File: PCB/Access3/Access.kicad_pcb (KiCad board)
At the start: 2 copper layers, 57.8 x 27 mm, 76 parts, among them J1 USB-C, J2 RFID, J3 INPUTS, J4 Shelly, J5 POWER, J6 DOOR2, J7 DOOR1, Q1 NX7002AK, Q2 PMF250XNEX, SW1 ESE13V01D, U1 ESP32-PICO-MINI-02, U2 FT231XQ, U3 G3VM-41GR8, U4 LMR16006XDDCR, U5 LMR16006XDDCR, U6 AA, U7 QR, U8 G3VM-41GR8, U9 AA

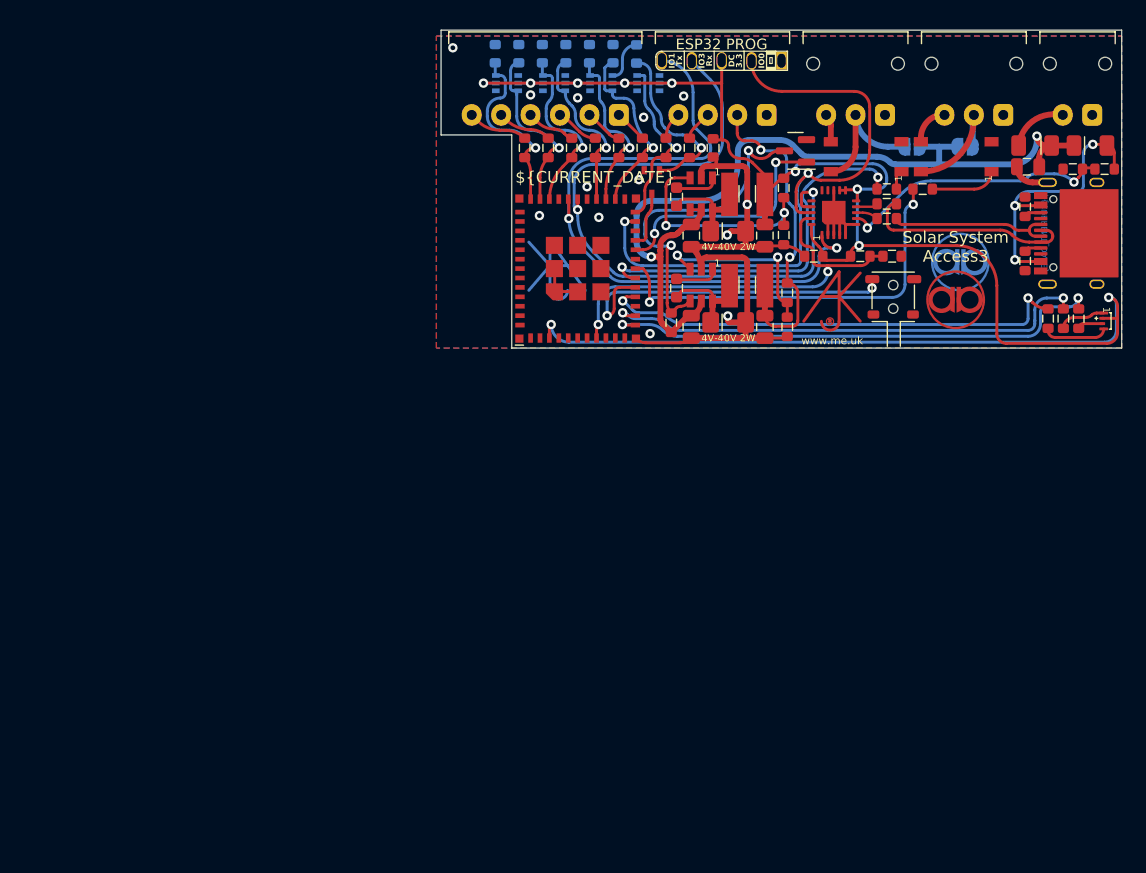
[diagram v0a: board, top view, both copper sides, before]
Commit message: Clean up
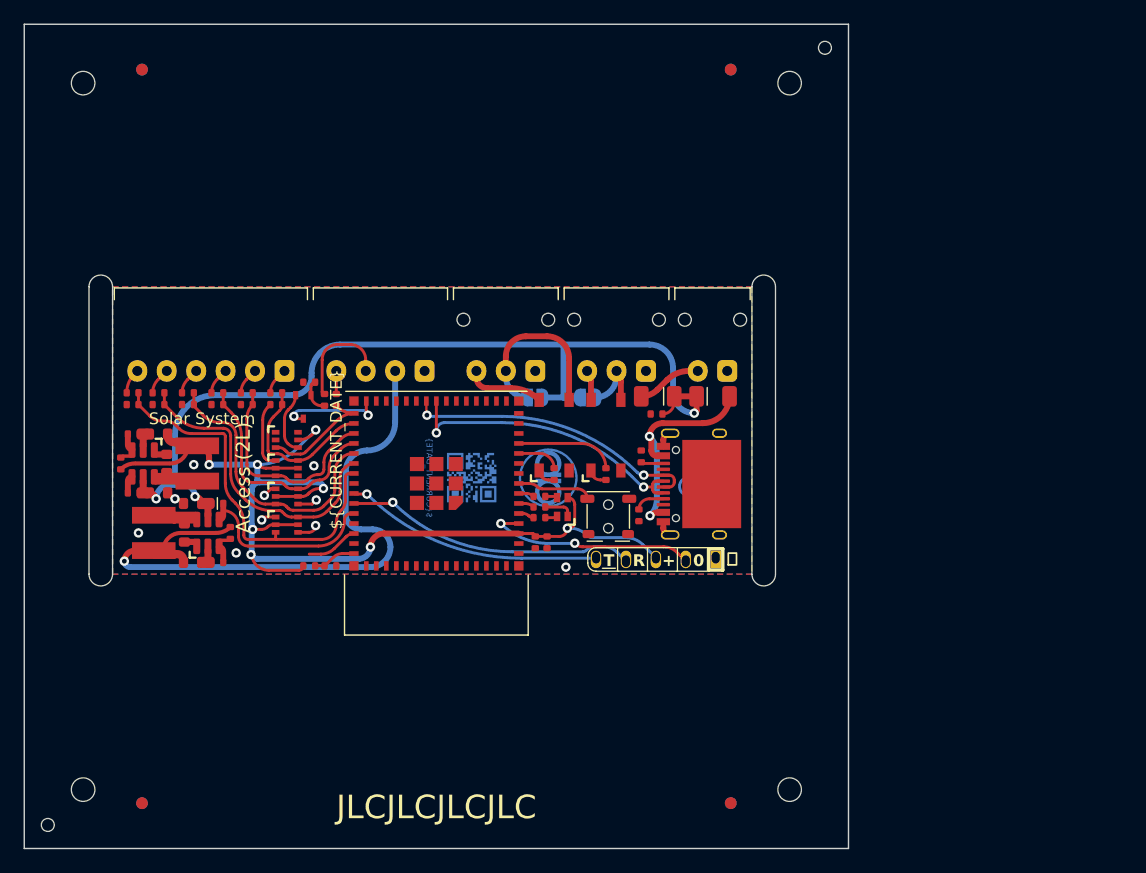
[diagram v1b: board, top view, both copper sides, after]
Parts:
- removed AJK1: AJK, RevK:AJK
- removed C10, C13: 2.2uF, RevK:C_0805_
- removed C11, C14: 10uF, RevK:C_0805_
- removed C12, C9: 100nF, RevK:C_0603_
- removed D5: LED_BARG, RevK:MHS190RGBCT
- removed D7: Schottky, RevK:D_1206_
- removed J4: Shelly, RevK:Shelly
- removed L1, L2: 6.8uH, RevK:L_4x4_
- removed Q1: NX7002AK, Package_TO_SOT_SMD:SOT-23
- removed R17: 300R, RevK:R_0603
- removed R18: 1K, RevK:R_0603
- removed R19: 100R, RevK:R_0603
- removed R22: 100k 1%, RevK:R_0603
- removed R23: 18k 1%, RevK:R_0603
- removed R24: 30k 1%, RevK:R_0603
- removed U4, U5: LMR16006XDDCR, RevK:SOT-23-Thin-6-Reg
- removed U6: AA, RevK:AA
- added C18: 100nF, RevK:C_0402, F.Cu at (108.4, 109.0)
- added C19: 22uF, RevK:C_0402, F.Cu at (109.4, 109.0)
- added C20: 1uF, RevK:C_0402, F.Cu at (91.0, 111.0)
- added C21: 10uF 50V, RevK:C_0603_, F.Cu at (76.6, 104.8)
- added C22: 10uF 6.3V, RevK:C_0603_, F.Cu at (76.4, 99.8)
- added C23: 100nF, RevK:C_0603_, F.Cu at (77.1, 102.3)
- added J8: Shelly, RevK:Shelly, F.Cu at (118.6, 110.5)
- added L3: 10uH, RevK:L_4x4_, F.Cu at (76.0, 108.2)
- added L4: 10uH, RevK:L_4x4_, F.Cu at (79.7, 102.3)
- added PCB1: 70x70, RevK:PCB7070, F.Cu at (100.0, 100.0)
- added R26: 10K, RevK:R_0402, F.Cu at (89.2, 111.0)
- added R27: 1M, RevK:R_0402_, F.Cu at (74.5, 104.8)
- added U10: ESP32-S3-MINI-1, RevK:ESP32-S3-MINI-1, F.Cu at (100.0, 104.0)
- added V1: ~, RevK:VCUT70, F.Cu at (100.0, 87.3)
- added V2: ~, RevK:VCUT70, F.Cu at (100.0, 111.7)
- C1: value 0.1uF -> 10uF 50V; footprint RevK:C_0603 -> RevK:C_0603_
- C15: value 1uF -> 10uF 6.3V; footprint RevK:C_0603 -> RevK:C_0603_
- C16: value 10nF -> 100nF; footprint RevK:C_0603 -> RevK:C_0603_
- C17: footprint RevK:C_0805 -> RevK:C_0402
- C2, C3, C4, C5, C6, C7, C8: footprint RevK:C_0603 -> RevK:C_0402; moved to F.Cu
- D1, D2, D3, D4: footprint Package_TO_SOT_SMD:SOT-363_SC-70-6 -> RevK:SOT-363_SC-70-6; moved to F.Cu
- D6: value Schottky -> RGB; footprint RevK:D_1206_ -> RevK:LED-RGB-1.6x1.6
- Logo1, U9: moved to B.Cu
- R1: value 10k -> 124k; footprint RevK:R_0603 -> RevK:R_0402_
- R10, R11, R12, R13, R16, R25, R4, R5, R6, R7, R8, R9: footprint RevK:R_0603 -> RevK:R_0402
- R14: value 27R -> 124k; footprint RevK:R_0603 -> RevK:R_0402_
- R15: value 27R -> 39k2; footprint RevK:R_0603 -> RevK:R_0402_
- R2: value 4k7 -> 23k2; footprint RevK:R_0603 -> RevK:R_0402_
- R20: value 100K -> 2K; footprint RevK:R_0603 -> RevK:R_0402
- R21: value 100k 1% -> 220R; footprint RevK:R_0603 -> RevK:R_0402
- R3: value 10k -> 680R; footprint RevK:R_0603 -> RevK:R_0402
- U1: value ESP32-PICO-MINI-02 -> MD8942; footprint RevK:ESP32-PICO-MINI-02 -> RevK:SOT-23-6-MD8942
- U2: value FT231XQ -> MD8942; footprint RevK:QFN-20-1EP_4x4mm_P0.5mm_EP2.5x2.5mm -> RevK:SOT-23-6-MD8942
- moved R2 82.4 mm to (81.4, 110.7)
- moved R14 68.7 mm to (73.2, 102.3), turned to 90 degrees
- moved R15 66.5 mm to (74.3, 99.8)
- moved C15 64.8 mm to (79.3, 110.7), turned to 0 degrees
- moved U2 62.4 mm to (75.1, 102.3)
- moved R1 58.4 mm to (82.5, 108.2), turned to -90 degrees
- moved C1 56.8 mm to (79.3, 105.7), turned to 0 degrees
- moved U7 56.2 mm to (103.0, 103.5)
- moved C16 55.5 mm to (78.6, 108.2)
- moved R3 53.6 mm to (108.8, 106.0)
- moved D1 43.1 mm to (87.3, 100.3)
- moved C8 42.9 mm to (74.2, 97.3), turned to 180 degrees
- moved C7 42.7 mm to (76.4, 97.3), turned to 180 degrees
- moved C6 42.4 mm to (78.9, 97.3), turned to 180 degrees
- moved D2 42.2 mm to (87.3, 102.7)
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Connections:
- J1 pad A6: Net-(J1-D+-PadA6) -> D+
- J1 pad A7: Net-(J1-D--PadA7) -> D-
- J1 pad B6: Net-(J1-D+-PadA6) -> D+
- J1 pad B7: Net-(J1-D--PadA7) -> D-
- R20 pad 1: Net-(Q1-D) -> Net-(D6-GK)
- R20 pad 2: +12V -> G
- R21 pad 1: +5V -> Net-(D6-BK)
- R21 pad 2: Net-(U4-FB) -> B
- R3 pad 1: Net-(U2-CBUS2) -> Net-(D6-RK)
- R3 pad 2: GND -> R
- U1 pad 1: GND -> unconnected-(U1-Pad1)
- U1 pad 3: +3.3V -> unconnected-(U1-Pad3)
- U1 pad 4: unconnected-(U1-I36-Pad4) -> SHDN
- U1 pad 5: unconnected-(U1-I37-Pad5) -> +12V
- U1 pad 7: unconnected-(U1-I39-Pad7) -> GND
- U1 pad 8: EN -> +5V
- U2 pad 1: O -> unconnected-(U2-Pad1)
- U2 pad 3: GND -> unconnected-(U2-Pad3)
- U2 pad 4: GND -> unconnected-(U2-EN-Pad4)
- U2 pad 5: GND -> +12V
- U2 pad 6: GND -> unconnected-(U2-Pad6)
- U2 pad 7: Net-(U2-CBUS2) -> GND
- U2 pad 8: D+ -> +3.3V
- U3 pad 3: Net-(J6-Pin_3) -> Net-(J6-Pin_2)
- U3 pad 4: Net-(J6-Pin_2) -> Net-(J6-Pin_3)
- U8 pad 3: Net-(J7-Pin_3) -> Net-(J7-Pin_2)
- U8 pad 4: Net-(J7-Pin_2) -> Net-(J7-Pin_3)
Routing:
- net +3.3V: track 156.1 -> 85.5 mm, vias 10 -> 8
- net I: track 58.5 -> 0.00 mm, vias 2 -> 0
- net O: track 57.1 -> 0.00 mm, vias 2 -> 0
- net BOOT: track 54.3 -> 0.00 mm, vias 2 -> 0
- net R: track 43.2 -> 1.33 mm, vias 2 -> 0
- net B: track 42.0 -> 1.31 mm, vias 2 -> 0
- net G: track 40.3 -> 1.30 mm, vias 2 -> 0
- net EN: track 35.8 -> 0.00 mm, vias 2 -> 0
- net RELAY2: track 32.1 -> 3.66 mm, vias 2 -> 0
- net Net-(Q1-D): track 27.5 -> 0.00 mm, vias 2 -> 0
- net RELAY1: track 34.5 -> 8.51 mm, vias 2 -> 0
- net Net-(J8-Rx): track 0.00 -> 24.7 mm, vias 0 -> 1
- net D-: track 1.53 -> 25.7 mm, vias 0 -> 2
- net D+: track 1.90 -> 25.1 mm, vias 0 -> 2
- net TAMPER: track 29.5 -> 6.38 mm, vias 2 -> 0
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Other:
- board size 57.8 x 27 mm -> 70 x 70 mm
- board text added: "3"
- board text added: "4"
- board text added: "6"
- board text added: "Access (2L)"
- board text added: "General I/O"
- board text added: "Solar System"
- board text added: "Solar System Access (2L)"
- board text removed: "-"
- board text removed: "Door Closed"
- board text removed: "Exit Button"
- board text removed: "General I/O 1-6"
- board text removed: "Lock Engaged"
- board text removed: "Power"
- board text removed: "Solar System Access3"
